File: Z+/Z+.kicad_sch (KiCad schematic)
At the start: 8 parts

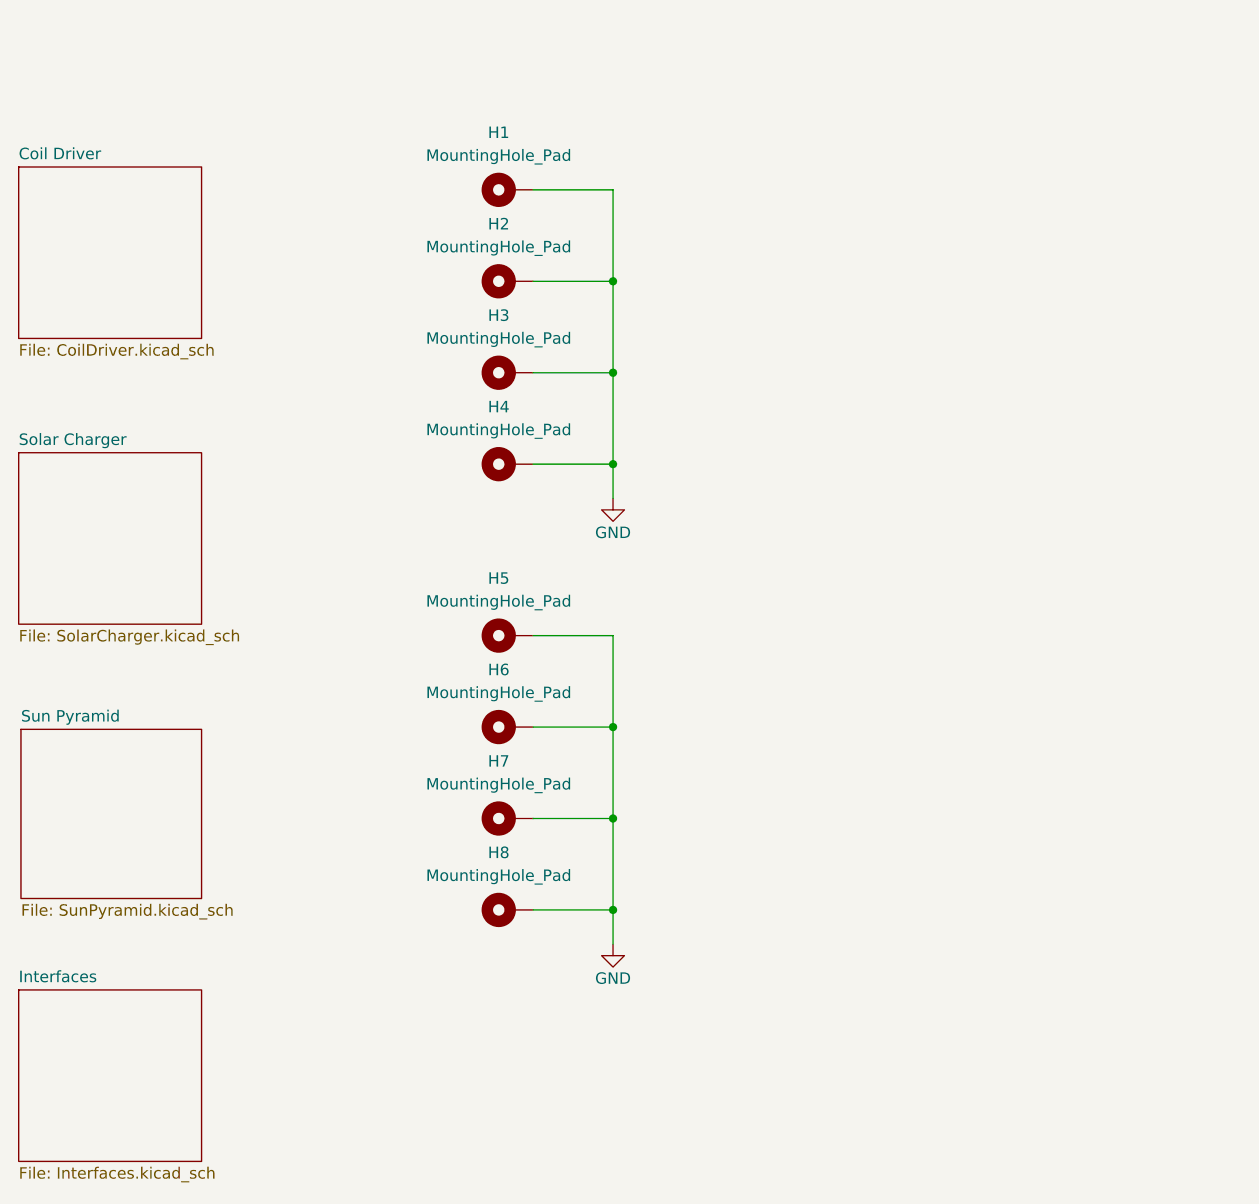
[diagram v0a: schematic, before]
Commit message: More layout work
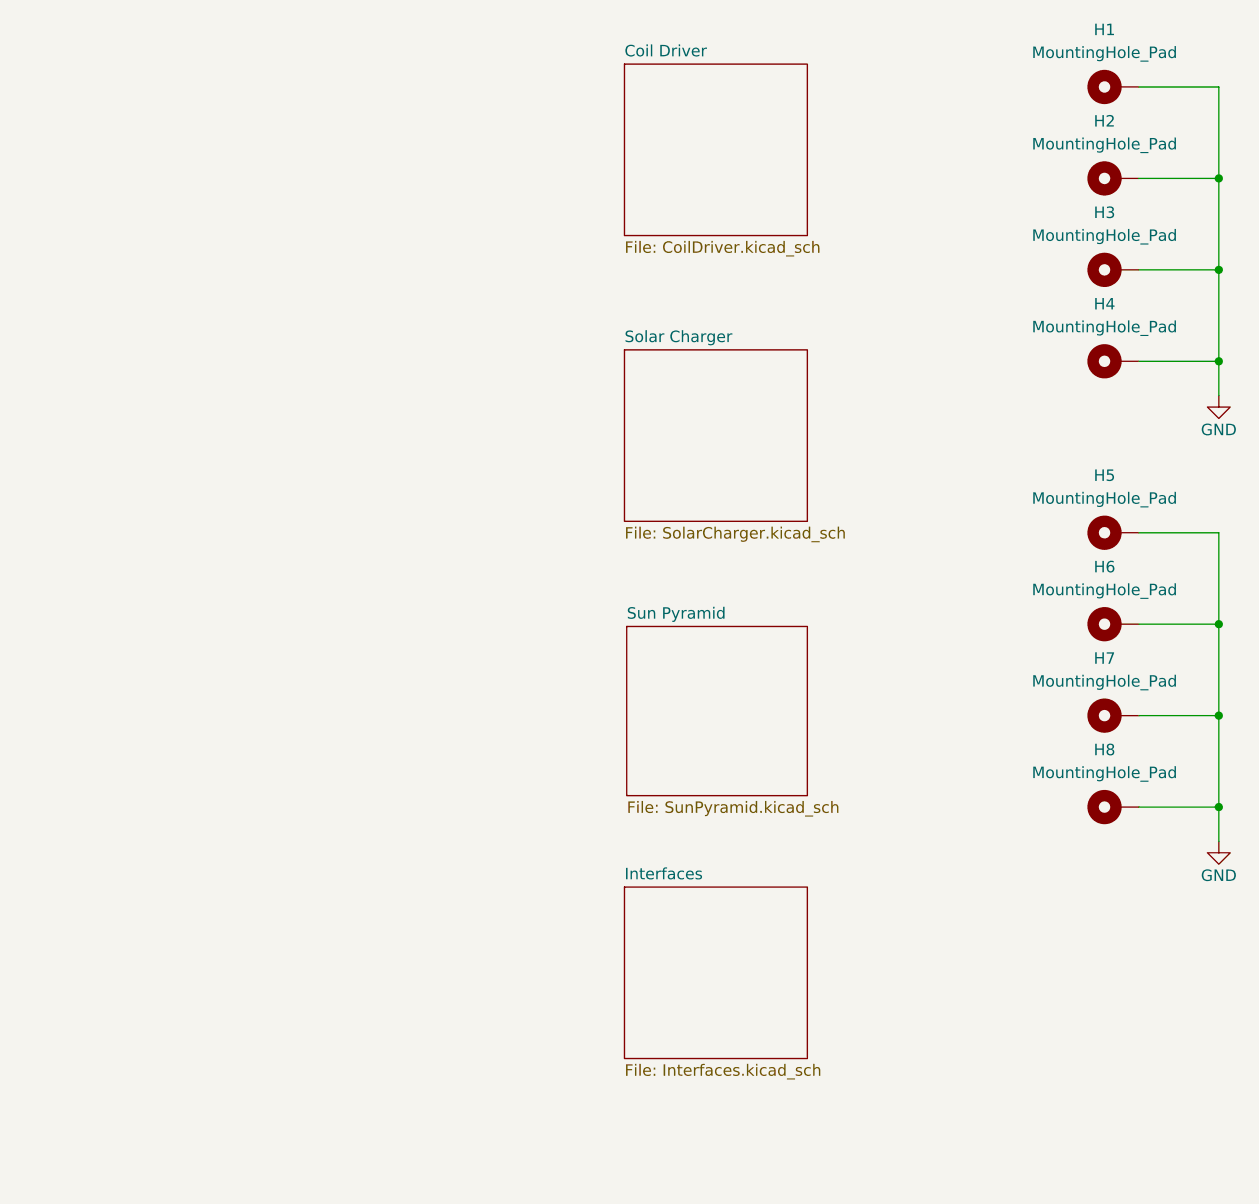
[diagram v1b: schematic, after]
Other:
- moved on the sheet: H1, H2, H3, H4, H5, H6, H7, H8
